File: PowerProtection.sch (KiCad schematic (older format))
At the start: 9 parts, among them K1 G6SK-2, Q1 IPB110P06LM

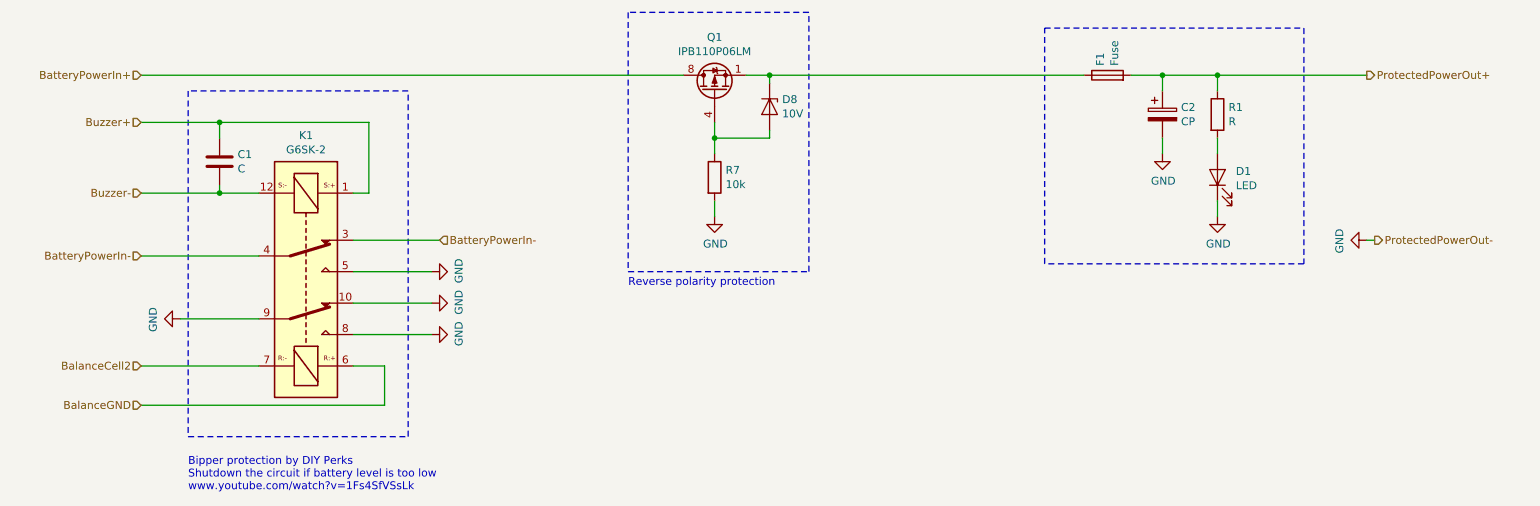
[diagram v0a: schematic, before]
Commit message: Fin du schema et routage
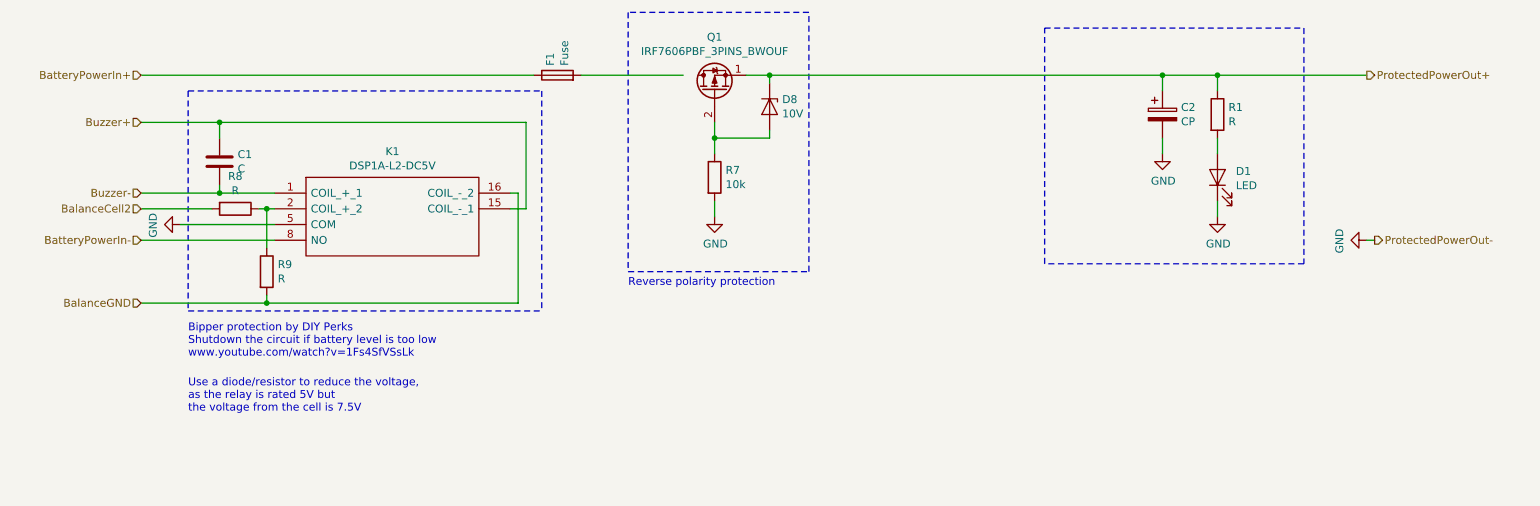
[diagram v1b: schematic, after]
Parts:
- removed K1: G6SK-2, symbol Relay:G6SK-2
- removed Q1: IPB110P06LM, Package_TO_SOT_SMD:TO-263-3_TabPin2, symbol Transistor_FET:IRF7606PBF
- added K1: DSP1A-L2-DC5V, SamacSys_Parts:DSP1AL2DC5V, symbol SamacSys_Parts:DSP1A-L2-DC5V
- added Q1: IRF7606PBF_3PINS_BWOUF, Package_TO_SOT_SMD:TO-263-3_TabPin2, symbol Transistor_FETvBwouf:IRF7606PBF_3PINS_BWOUF
- added R8, R9: R, LIB_BE_PHELMA_CMS:R_1206_3216Metric_Pad1.42x1.75mm_HandSolder, symbol Device:R
- D8: footprint (none) -> LIB_BE_PHELMA_CMS:LED_1206_3216Metric_Pad1.42x1.75mm_HandSolder
- F1: footprint (none) -> Fuse:Fuse_1210_3225Metric_Pad1.42x2.65mm_HandSolder
- R7: footprint (none) -> LIB_BE_PHELMA_CMS:R_1206_3216Metric_Pad1.42x1.75mm_HandSolder
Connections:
- net BalanceCell2: now also R8.2
- net BalanceGND: now also K1.16 (COIL_-_2), R9.2
- net BatteryPowerIn+: now also F1.1
- net BatteryPowerIn-: now also K1.8 (NO)
- net Buzzer+: now also K1.15 (COIL_-_1)
- net Buzzer-: now also K1.1 (COIL_+_1)
- net GND: now also K1.5 (COM)
- net ProtectedPowerOut+: now also D8.1 (K), Q1.1 (S); no longer F1.2
- net at D8.2 (A), R7.1: now also Q1.2 (G)
- new net: F1.2, Q1.3 (D)
- new net: K1.2 (COIL_+_2), R8.1, R9.1
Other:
- note added: "Use a diode/resistor to reduce the voltage,\nas the relay is rated 5V but \nthe voltage from the cell is 7.5V\n"
- moved on the sheet: F1
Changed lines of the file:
@@
 Wire Wire Line
 	8750 3050 8750 3150
-Wire Wire Line
-	8550 3050 8750 3050
 $Comp
 L power:GND #PWR?
@@
 L Device:Fuse F?
 U 1 1 5F823127
-P 8400 3050
+P 4900 3050
 AR Path="/5F823127" Ref="F?"  Part="1"
 AR Path="/5F802FB9/5F823127" Ref="F1"  Part="1"
-F 0 "F1" H 8460 3096 50  0000 L CNN
-F 1 "Fuse" H 8460 3005 50  0000 L CNN
-F 2 "" V 8330 3050 50  0001 C CNN
-F 3 "~" H 8400 3050 50  0001 C CNN
-	1    8400 3050
+F 0 "F1" H 4960 3096 50  0000 L CNN
+F 1 "Fuse" H 4960 3005 50  0000 L CNN
+F 2 "Fuse:Fuse_1210_3225Metric_Pad1.42x2.65mm_HandSolder" V 4830 3050 50  0001 C CNN
+F 3 "~" H 4900 3050 50  0001 C CNN
+	1    4900 3050
 	0    -1   -1   0
 $EndComp
 Text HLabel 10050 3050 2    50   Output ~ 0
 ProtectedPowerOut+
-$Comp
-L Relay:G6SK-2 K1
-U 1 1 5F83DBFF
-P 3300 4300
-F 0 "K1" V 2433 4300 50  0000 C CNN
-F 1 "G6SK-2" V 2524 4300 50  0000 C CNN
-F 2 "" H 3850 4250 50  0001 L CNN
-F 3 "http://omronfs.omron.com/en_US/ecb/products/pdf/en-g6s.pdf" H 3000 4300 50  0001 C CNN
-	1    3300 4300
-	0    1    1    0
-$EndComp
-Text HLabel 2250 4200 0    50   Input ~ 0
+Text HLabel 2250 4100 0    50   Input ~ 0
 BatteryPowerIn-
-Text HLabel 10100 4100 2    50   Output ~ 0
-ProtectedPowerOut-
 $Comp
 L Device:C C1
@@
 Buzzer+
 Wire Wire Line
-	3600 4900 3800 4900
-Wire Wire Line
-	3800 4900 3800 5150
-Wire Wire Line
-	3700 3800 3700 3350
-Wire Wire Line
-	3700 3350 2750 3350
-Wire Wire Line
 	2750 3350 2750 3450
-Wire Wire Line
-	3600 3800 3700 3800
-Wire Wire Line
-	3000 3800 2750 3800
 Wire Wire Line
 	2750 3800 2750 3750
@@
 Wire Wire Line
 	2250 3800 2750 3800
-Wire Wire Line
-	2250 4200 3000 4200
-Text HLabel 2250 4900 0    50   Input ~ 0
-BalanceCell2
-Text HLabel 2250 5150 0    50   Input ~ 0
+Text HLabel 2250 4500 0    50   Input ~ 0
 BalanceGND
-Wire Wire Line
-	2250 4900 3000 4900
-Wire Wire Line
-	2250 5150 3800 5150
-Wire Notes Line
-	2550 3150 2550 5350
-Wire Notes Line
-	2550 5350 3950 5350
-Wire Notes Line
-	3950 5350 3950 3150
-Wire Notes Line
-	3950 3150 2550 3150
-Text Notes 2550 5700 0    50   ~ 0
+Text Notes 2550 4850 0    50   ~ 0
 Bipper protection by DIY Perks\nShutdown the circuit if battery level is too low\nwww.youtube.com/watch?v=1Fs4SfVSsLk
-Wire Wire Line
-	3600 4300 4100 4300
 $Comp
 L power:GND #PWR?
 U 1 1 5FAC711C
-P 2500 4600
+P 2500 4000
 AR Path="/5FAC711C" Ref="#PWR?"  Part="1"
 AR Path="/5F802FB9/5FAC711C" Ref="#PWR0101"  Part="1"
-F 0 "#PWR0101" H 2500 4350 50  0001 C CNN
-F 1 "GND" H 2505 4427 50  0000 C CNN
-F 2 "" H 2500 4600 50  0001 C CNN
-F 3 "" H 2500 4600 50  0001 C CNN
-	1    2500 4600
+F 0 "#PWR0101" H 2500 3750 50  0001 C CNN
+F 1 "GND" H 2505 3827 50  0000 C CNN
+F 2 "" H 2500 4000 50  0001 C CNN
+F 3 "" H 2500 4000 50  0001 C CNN
+	1    2500 4000
 	0    1    1    0
-$EndComp
-$Comp
-L power:GND #PWR?
-U 1 1 5FAC7686
-P 4100 4700
-AR Path="/5FAC7686" Ref="#PWR?"  Part="1"
-AR Path="/5F802FB9/5FAC7686" Ref="#PWR0102"  Part="1"
-F 0 "#PWR0102" H 4100 4450 50  0001 C CNN
-F 1 "GND" H 4105 4527 50  0000 C CNN
-F 2 "" H 4100 4700 50  0001 C CNN
-F 3 "" H 4100 4700 50  0001 C CNN
-	1    4100 4700
-	0    -1   -1   0
-$EndComp
-$Comp
-L power:GND #PWR?
-U 1 1 5FAC7C37
-P 4100 4500
-AR Path="/5FAC7C37" Ref="#PWR?"  Part="1"
-AR Path="/5F802FB9/5FAC7C37" Ref="#PWR0103"  Part="1"
-F 0 "#PWR0103" H 4100 4250 50  0001 C CNN
-F 1 "GND" H 4105 4327 50  0000 C CNN
-F 2 "" H 4100 4500 50  0001 C CNN
-F 3 "" H 4100 4500 50  0001 C CNN
-	1    4100 4500
-	0    -1   -1   0
-$EndComp
-Text HLabel 4150 4100 2    50   Input ~ 0
-BatteryPowerIn-
-Wire Wire Line
-	3600 4100 4150 4100
-$Comp
-L power:GND #PWR?
-U 1 1 5F8A11CB
-P 4100 4300
-AR Path="/5F8A11CB" Ref="#PWR?"  Part="1"
-AR Path="/5F802FB9/5F8A11CB" Ref="#PWR0105"  Part="1"
-F 0 "#PWR0105" H 4100 4050 50  0001 C CNN
-F 1 "GND" H 4105 4127 50  0000 C CNN
-F 2 "" H 4100 4300 50  0001 C CNN
-F 3 "" H 4100 4300 50  0001 C CNN
-	1    4100 4300
-	0    -1   -1   0
-$EndComp
-$Comp
-L power:GND #PWR?
-U 1 1 5F8A37D8
-P 10050 4100
-AR Path="/5F8A37D8" Ref="#PWR?"  Part="1"
-AR Path="/5F802FB9/5F8A37D8" Ref="#PWR0106"  Part="1"
-F 0 "#PWR0106" H 10050 3850 50  0001 C CNN
-F 1 "GND" H 10055 3927 50  0000 C CNN
-F 2 "" H 10050 4100 50  0001 C CNN
-F 3 "" H 10050 4100 50  0001 C CNN
-	1    10050 4100
-	0    1    1    0
-$EndComp
-Wire Wire Line
-	10100 4100 10050 4100
-Wire Wire Line
-	2500 4600 3000 4600
-Wire Wire Line
-	3600 4700 4100 4700
-Wire Wire Line
-	3600 4500 4100 4500
-$Comp
-L Transistor_FET:IRF7606PBF Q?
-U 1 1 5F88E169
-P 5900 3150
-AR Path="/5F88E169" Ref="Q?"  Part="1"
-AR Path="/5F898EC7/5F88E169" Ref="Q?"  Part="1"
-AR Path="/5F802FB9/5FBB308A/5F88E169" Ref="Q?"  Part="1"
-AR Path="/5F802FB9/5F88E169" Ref="Q1"  Part="1"
-F 0 "Q1" V 6242 3150 50  0000 C CNN
-F 1 "IPB110P06LM" V 6151 3150 50  0000 C CNN
-F 2 "Package_TO_SOT_SMD:TO-263-3_TabPin2" H 6100 3075 50  0001 L CIN
-F 3 "https://www.infineon.com/dgdl/Infineon-IPB110P06LM-DS-v02_00-EN.pdf?fileId=5546d46269e1c019016a03e2d06000ae" V 5900 3150 50  0001 L CNN
-	1    5900 3150
-	0    -1   -1   0
 $EndComp
 $Comp
@@
 F 0 "D8" V 6204 3330 50  0000 L CNN
 F 1 "10V" V 6295 3330 50  0000 L CNN
-F 2 "" H 6250 3250 50  0001 C CNN
+F 2 "LIB_BE_PHELMA_CMS:LED_1206_3216Metric_Pad1.42x1.75mm_HandSolder" H 6250 3250 50  0001 C CNN
 F 3 "~" H 6250 3250 50  0001 C CNN
 	1    6250 3250
@@
 F 0 "R7" H 5970 3746 50  0000 L CNN
 F 1 "10k" H 5970 3655 50  0000 L CNN
-F 2 "" V 5830 3700 50  0001 C CNN
+F 2 "LIB_BE_PHELMA_CMS:R_1206_3216Metric_Pad1.42x1.75mm_HandSolder" V 5830 3700 50  0001 C CNN
 F 3 "~" H 5900 3700 50  0001 C CNN
 	1    5900 3700
@@
 	6250 3100 6250 3050
 Connection ~ 6250 3050
-Wire Wire Line
-	2250 3050 5700 3050
-Wire Wire Line
-	6250 3050 8250 3050
 Wire Notes Line
 	5350 2650 5350 4300
@@
 Wire Wire Line
 	9100 3050 10050 3050
+$Comp
+L Transistor_FETvBwouf:IRF7606PBF_3PINS_BWOUF Q1
+U 1 1 5F9E94BA
+P 5900 3150
+F 0 "Q1" V 6243 3150 50  0000 C CNN
+F 1 "IRF7606PBF_3PINS_BWOUF" V 6152 3150 50  0000 C CNN
+F 2 "Package_TO_SOT_SMD:TO-263-3_TabPin2" H 6100 3075 50  0001 L CIN
+F 3 "http://www.irf.com/product-info/datasheets/data/irf7606pbf.pdf" V 5900 3150 50  0001 L CNN
+	1    5900 3150
+	0    -1   -1   0
+$EndComp
+Wire Wire Line
+	2250 3050 4750 3050
+Wire Wire Line
+	5050 3050 5700 3050
+Text HLabel 2250 3900 0    50   Input ~ 0
+BalanceCell2
+Wire Wire Line
+	6250 3050 8750 3050
+$Comp
+L power:GND #PWR?
+U 1 1 5F8A37D8
+P 10050 4100
+AR Path="/5F8A37D8" Ref="#PWR?"  Part="1"
+AR Path="/5F802FB9/5F8A37D8" Ref="#PWR0106"  Part="1"
+F 0 "#PWR0106" H 10050 3850 50  0001 C CNN
+F 1 "GND" H 10055 3927 50  0000 C CNN
+F 2 "" H 10050 4100 50  0001 C CNN
+F 3 "" H 10050 4100 50  0001 C CNN
+	1    10050 4100
+	0    1    1    0
+$EndComp
+Wire Wire Line
+	10100 4100 10050 4100
+Text HLabel 10100 4100 2    50   Output ~ 0
+ProtectedPowerOut-
+Wire Wire Line
+	4700 3350 4700 3900
+Wire Wire Line
+	2750 3350 4700 3350
+Wire Notes Line
+	2550 4550 4800 4550
+Wire Notes Line
+	2550 3150 4800 3150
+Wire Wire Line
+	2700 3900 2250 3900
+Text Notes 2550 5200 0    50   ~ 0
+Use a diode/resistor to reduce the voltage,\nas the relay is rated 5V but \nthe voltage from the cell is 7.5V\n
+Wire Wire Line
+	4650 3800 4600 3800
+$Comp
+L SamacSys_Parts:DSP1A-L2-DC5V K1
+U 1 1 5FA57E7A
+P 3100 3800
+F 0 "K1" H 3850 4065 50  0000 C CNN
+F 1 "DSP1A-L2-DC5V" H 3850 3974 50  0000 C CNN
+F 2 "SamacSys_Parts:DSP1AL2DC5V" H 4450 3900 50  0001 L CNN
+F 3 "https://componentsearchengine.com/Datasheets/1/DSP1A-L2-DC5V.pdf" H 4450 3800 50  0001 L CNN
+F 4 "General Purpose Relays 8A 5VDC SPST 2 COIL LATCHING PCB" H 4450 3700 50  0001 L CNN "Description"
+F 5 "10.8" H 4450 3600 50  0001 L CNN "Height"
+F 6 "769-DSP1A-L2-DC5V" H 4450 3500 50  0001 L CNN "Mouser Part Number"
+F 7 "https://www.mouser.com/Search/Refine.aspx?Keyword=769-DSP1A-L2-DC5V" H 4450 3400 50  0001 L CNN "Mouser Price/Stock"
+F 8 "Panasonic" H 4450 3300 50  0001 L CNN "Manufacturer_Name"
+F 9 "DSP1A-L2-DC5V" H 4450 3200 50  0001 L CNN "Manufacturer_Part_Number"
+	1    3100 3800
+	1    0    0    -1
+$EndComp
+Wire Wire Line
+	4700 3900 4600 3900
+Wire Wire Line
+	2750 3800 3100 3800
+$Comp
+L Device:R R8
+U 1 1 5FADC1E8
+P 2850 3900
+F 0 "R8" V 2643 3900 50  0000 C CNN
+F 1 "R" V 2734 3900 50  0000 C CNN
+F 2 "LIB_BE_PHELMA_CMS:R_1206_3216Metric_Pad1.42x1.75mm_HandSolder" V 2780 3900 50  0001 C CNN
+F 3 "~" H 2850 3900 50  0001 C CNN
+	1    2850 3900
+	0    1    1    0
+$EndComp
+Wire Wire Line
+	2500 4000 3100 4000
+Wire Wire Line
+	2250 4100 3100 4100
+$Comp
+L Device:R R9
+U 1 1 5FADE5C8
+P 3050 4300
+F 0 "R9" H 3120 4346 50  0000 L CNN
+F 1 "R" H 3120 4255 50  0000 L CNN
+F 2 "LIB_BE_PHELMA_CMS:R_1206_3216Metric_Pad1.42x1.75mm_HandSolder" V 2980 4300 50  0001 C CNN
+F 3 "~" H 3050 4300 50  0001 C CNN
+	1    3050 4300
+	1    0    0    -1
+$EndComp
+Wire Wire Line
+	3000 3900 3050 3900
+Wire Wire Line
+	2250 4500 3050 4500
+Wire Notes Line
+	4800 3150 4800 4550
+Wire Notes Line
+	2550 3150 2550 4550
+Wire Wire Line
+	4650 3800 4650 4500
+Wire Wire Line
+	3050 4450 3050 4500
+Connection ~ 3050 4500
+Wire Wire Line
+	3050 4500 4650 4500
+Wire Wire Line
+	3050 4150 3050 3900
+Connection ~ 3050 3900
+Wire Wire Line
+	3050 3900 3100 3900
 $EndSCHEMATC

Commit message: Avec regul moteur et texte sur autre couche
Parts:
- Q1: footprint Package_TO_SOT_SMD:TO-263-3_TabPin2 -> Package_TO_SOT_SMD:TO-252-3_TabPin2
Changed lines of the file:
@@
 F 0 "Q1" V 6243 3150 50  0000 C CNN
 F 1 "IRF7606PBF_3PINS_BWOUF" V 6152 3150 50  0000 C CNN
-F 2 "Package_TO_SOT_SMD:TO-263-3_TabPin2" H 6100 3075 50  0001 L CIN
+F 2 "Package_TO_SOT_SMD:TO-252-3_TabPin2" H 6100 3075 50  0001 L CIN
 F 3 "http://www.irf.com/product-info/datasheets/data/irf7606pbf.pdf" V 5900 3150 50  0001 L CNN
 	1    5900 3150
@@
 Wire Wire Line
 	2700 3900 2250 3900
-Text Notes 2550 5200 0    50   ~ 0
-Use a diode/resistor to reduce the voltage,\nas the relay is rated 5V but \nthe voltage from the cell is 7.5V\n
 Wire Wire Line
 	4650 3800 4600 3800
@@
 Wire Wire Line
 	3050 3900 3100 3900
+Text Notes 2550 5200 0    50   ~ 0
+Use a diode/resistor to reduce the voltage,\nas the relay is rated 5V but \nthe voltage from the cell is 7.5V\n
 $EndSCHEMATC
